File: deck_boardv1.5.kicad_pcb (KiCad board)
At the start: 4 copper layers, 89.2 x 41.3 mm, 56 parts, among them J1 430450800, J2 Conn_01x01_Pin, J3 Conn_01x01_Pin, J4 Conn_01x01_Pin, J5 Conn_01x01_Pin, J6 Conn_01x01_Pin, J7 Conn_01x01_Pin, Q1 MMBT3904, Q2 2N7002, Q3 NMOS, U1 Raspberry Pi Zero 2 W, U2 LT8610AC, U3 DIGI XBee-PRO 900HP RF Module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, U4 ADP7158ARDZ-3.3-R7

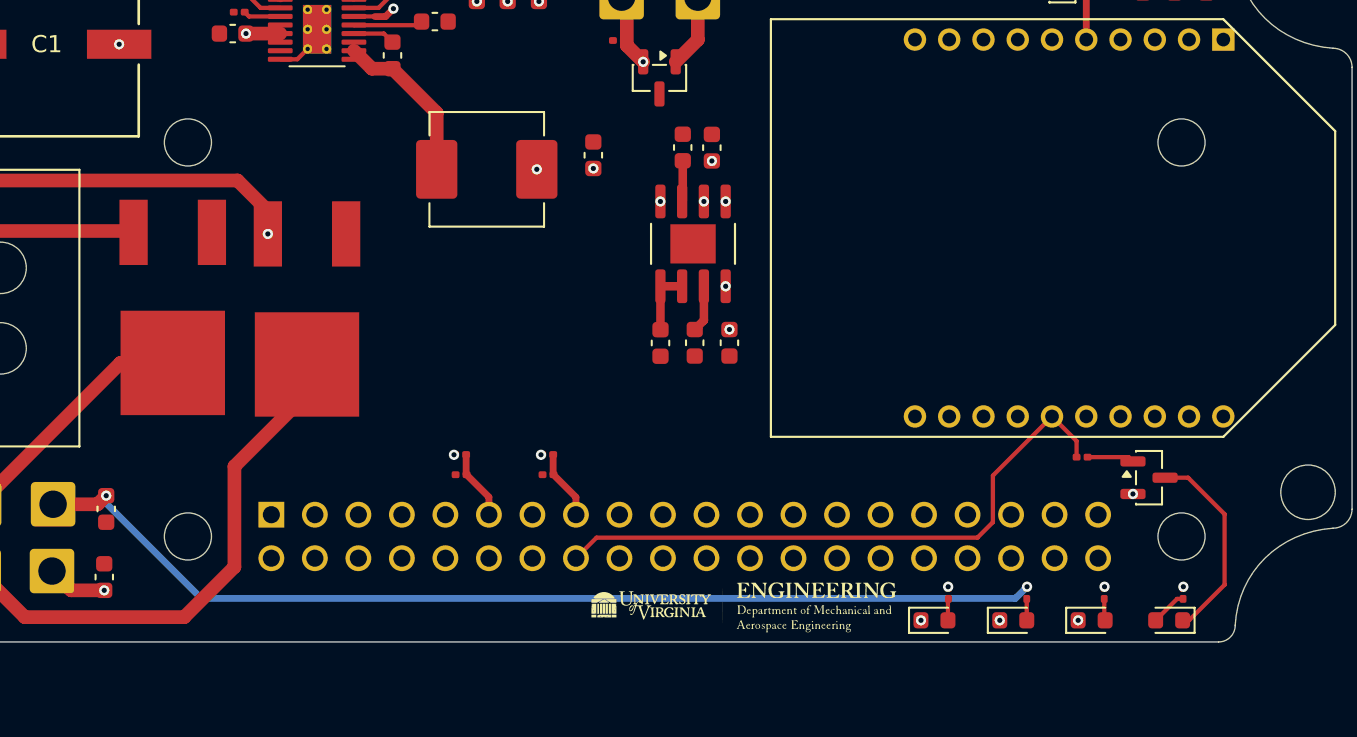
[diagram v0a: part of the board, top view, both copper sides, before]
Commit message: Adjusted components.
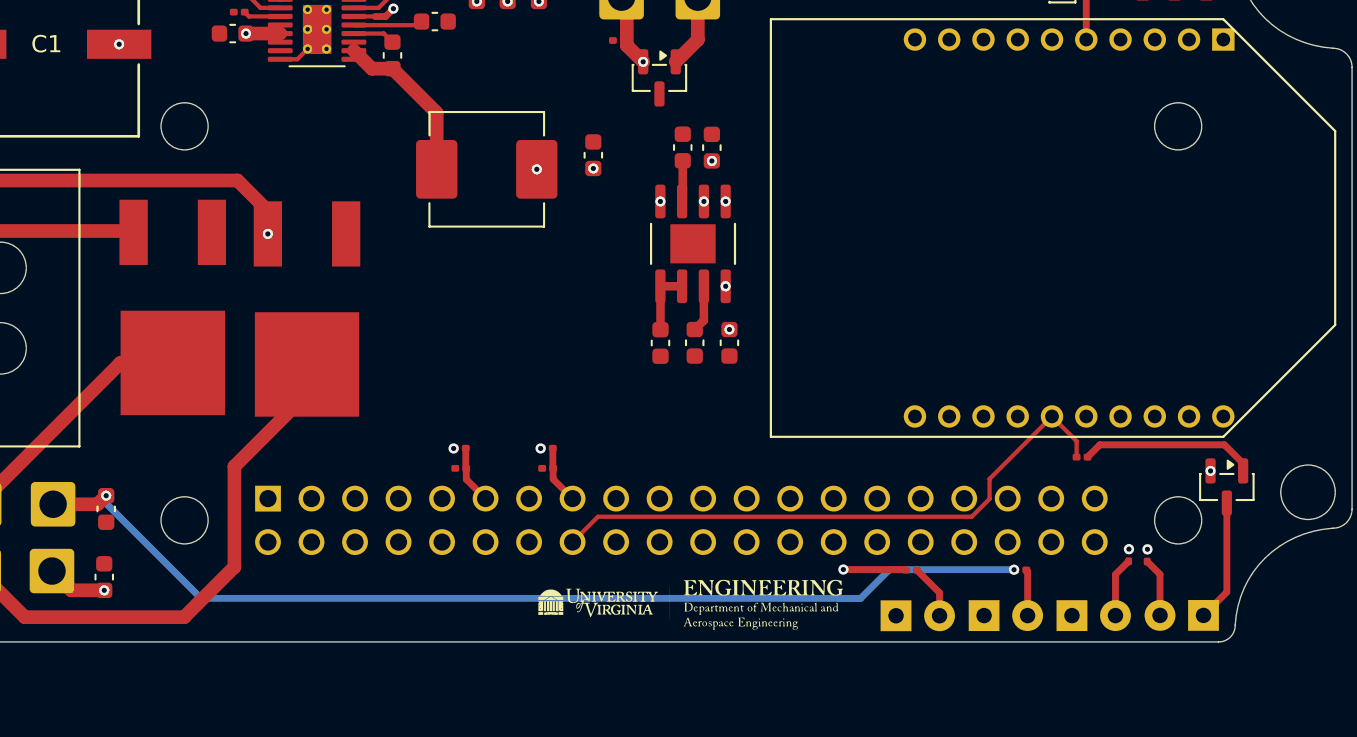
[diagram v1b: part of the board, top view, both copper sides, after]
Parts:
- D2, D4, D5, D6: footprint LED_SMD:LED_0603_1608Metric -> LED_THT:LED_D3.0mm
- moved Q1 4.57 mm to (184.6, 91.4), turned to -90 degrees
- moved G*** 3.10 mm to (153.3, 98.3)
- moved R6 3.03 mm to (179.9, 95.4)
- moved R5 2.62 mm to (178.8, 95.4)
- moved R14 2.54 mm to (166.2, 96.2), turned to 0 degrees
- moved D6 2.26 mm to (165.3, 98.9)
- moved D5 2.03 mm to (183.2, 98.9)
- moved D2 1.72 mm to (170.4, 98.9)
- moved R13 1.41 mm to (172.6, 96.2), turned to 180 degrees
- moved D4 1.18 mm to (175.5, 98.9)
- moved U1 0.96 mm to (152.7, 81.8)
- moved R12 0.37 mm to (144.9, 89.1)
- moved R9 0.37 mm to (139.8, 89.1)
- moved R11 0.37 mm to (144.9, 90.3)
- moved R10 0.37 mm to (139.9, 90.3)
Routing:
- net Net-(Q1-B): track 2.75 -> 10.3 mm
- net Net-(D5-K): track 11.8 -> 7.12 mm
- net GPIO15: track 56.7 -> 60.3 mm
- net Net-(D4-A): track 1.27 -> 3.49 mm
- net Net-(D6-A): track 1.26 -> 3.20 mm
- net Net-(D2-A): track 1.25 -> 2.62 mm
- net Net-(D5-A): track 2.12 -> 3.46 mm
- net XBee_ASSOC: track 35.8 -> 34.7 mm
- net ENABLE: track 102.0 -> 100.9 mm
- net GPIO24: track 51.9 -> 51.0 mm
- net Net-(U1-GPIO22/GPIO_GEN3): track 4.07 -> 3.39 mm
- net Net-(U1-GPIO17/GPIO_GEN0): track 4.06 -> 3.38 mm
- net GND: vias 4 -> 1
